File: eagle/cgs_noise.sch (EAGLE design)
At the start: 18 parts, among them IC1 TL074P, Q1 2N3906, Q2 2N3906

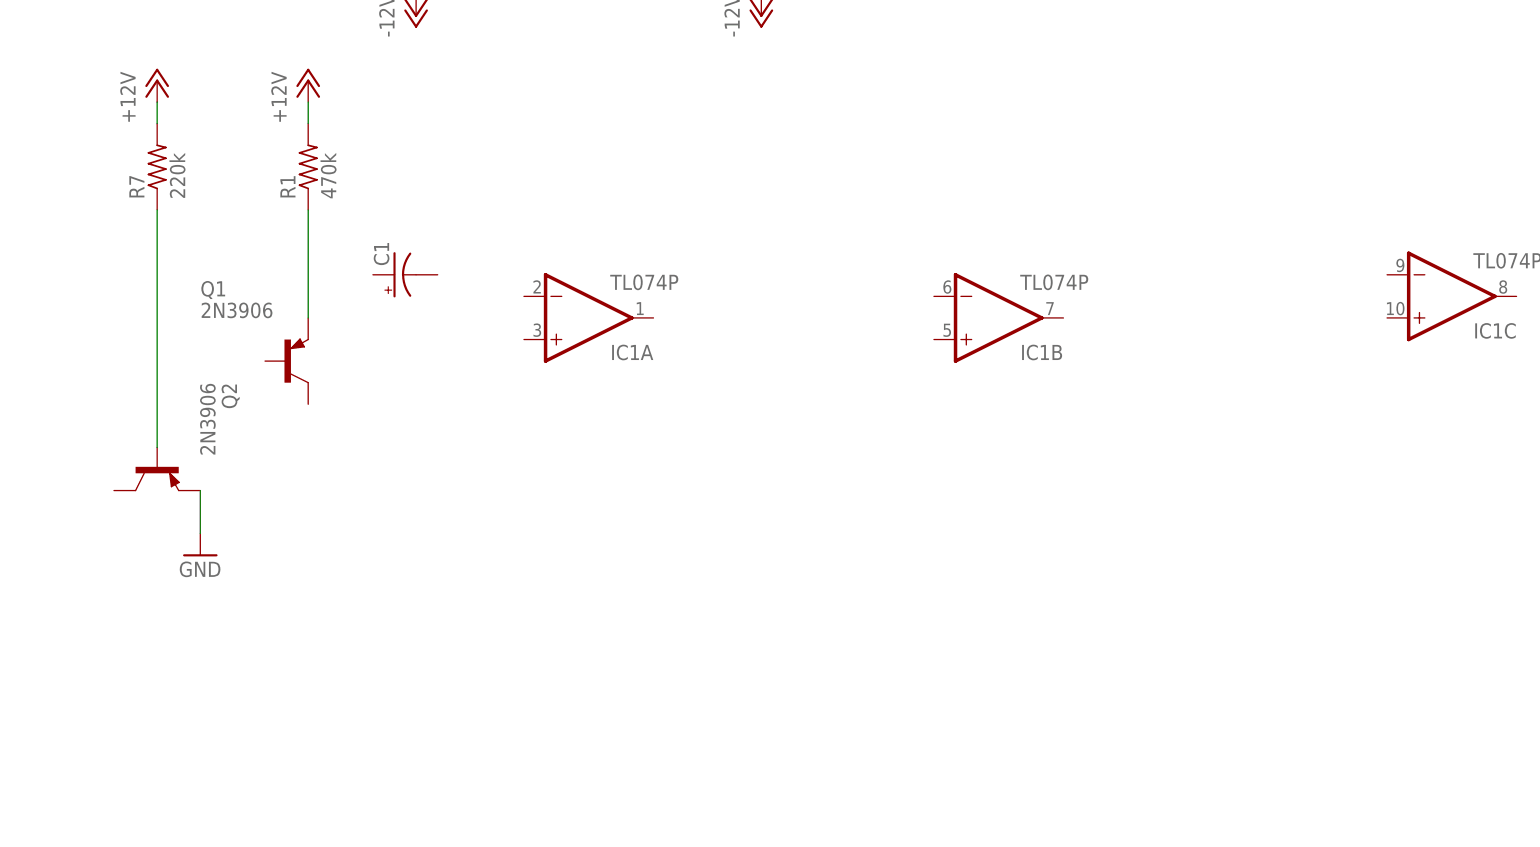
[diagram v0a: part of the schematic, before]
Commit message: initial commit
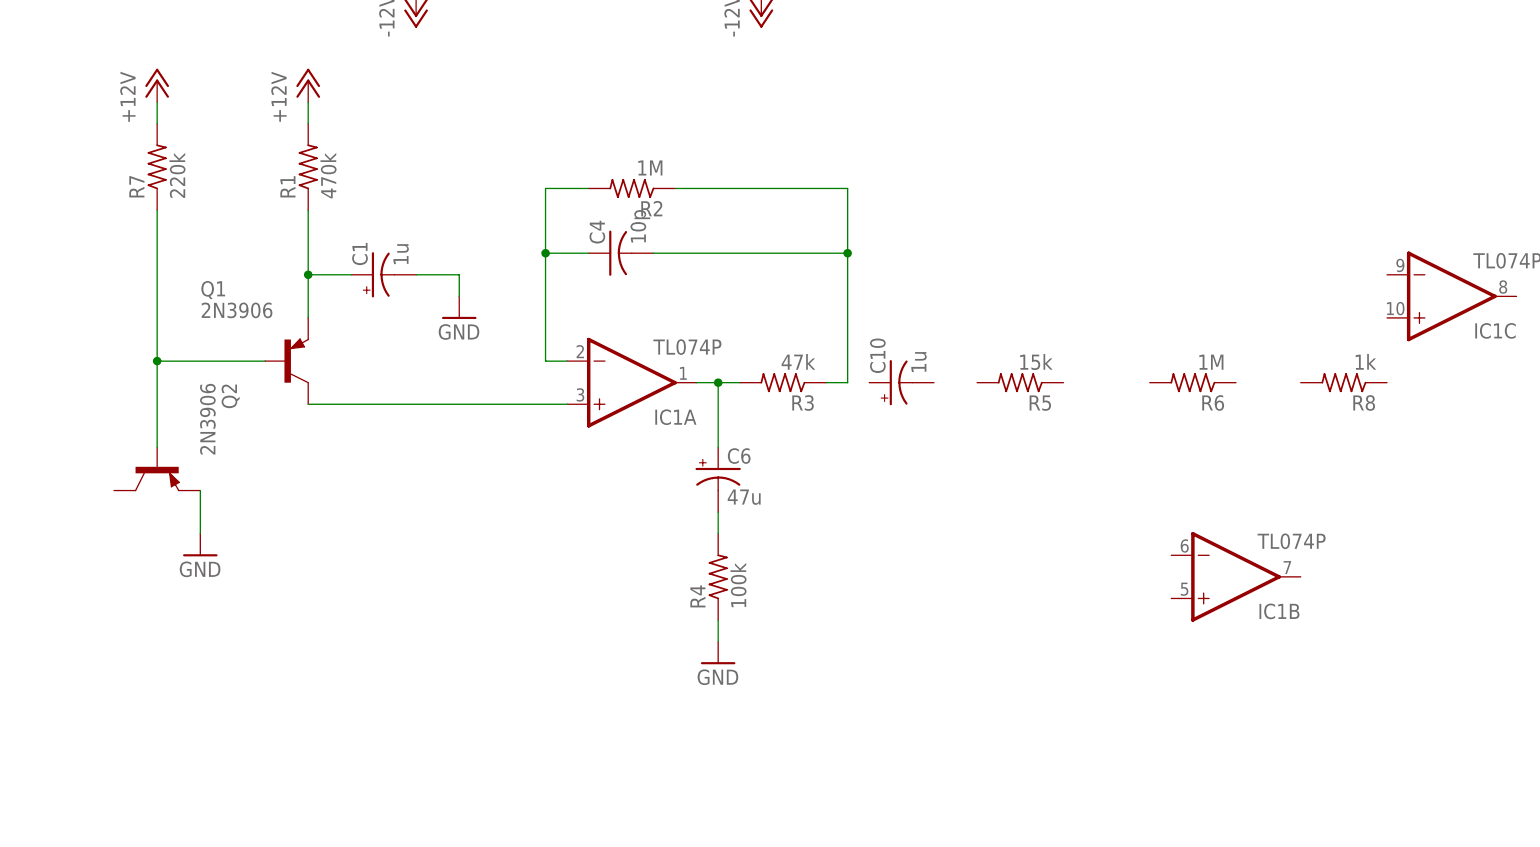
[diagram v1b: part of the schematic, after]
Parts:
- added C10: 1u, rcl:CPOL-USB45181A
- added C4: 10p, rcl:C-US050-024X044
- added C6: 47u, rcl:CPOL-USB45181A
- added R2, R6: 1M, rcl:R-US_0207/10
- added R3: 47k, rcl:R-US_0207/10
- added R4: 100k, rcl:R-US_0207/10
- added R5: 15k, rcl:R-US_0207/10
- added R8: 1k, rcl:R-US_0207/10
- C1: value (none) -> 1u
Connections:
- new net N$3: IC1A.+IN, Q1.C
- new net N$4: C6.+, IC1A.OUT, R3.2
- new net N$5: C6.-, R4.2
- new net N$6: C4.2, R2.1, R3.1
- new net N$7: C4.1, IC1A.-IN, R2.2
- net GND: now also C1.-, R4.1
- net N$1: now also C1.+
- net N$2: now also Q1.B
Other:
- moved on the sheet: C1, IC1A, IC1B
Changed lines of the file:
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@@
 <part name="Q2" library="transistor-pnp" deviceset="2N3906" device=""/>
 <part name="GND2" library="supply1" deviceset="GND" device=""/>
-<part name="C1" library="rcl" deviceset="CPOL-US" device="B45181A"/>
+<part name="C1" library="rcl" deviceset="CPOL-US" device="B45181A" value="1u"/>
+<part name="GND3" library="supply1" deviceset="GND" device=""/>
+<part name="R2" library="rcl" deviceset="R-US_" device="0207/10" value="1M"/>
+<part name="C4" library="rcl" deviceset="C-US" device="050-024X044" value="10p"/>
+<part name="R3" library="rcl" deviceset="R-US_" device="0207/10" value="47k"/>
+<part name="C6" library="rcl" deviceset="CPOL-US" device="B45181A" value="47u"/>
+<part name="R4" library="rcl" deviceset="R-US_" device="0207/10" value="100k"/>
+<part name="GND4" library="supply1" deviceset="GND" device=""/>
+<part name="C10" library="rcl" deviceset="CPOL-US" device="B45181A" value="1u"/>
+<part name="R5" library="rcl" deviceset="R-US_" device="0207/10" value="15k"/>
+<part name="R6" library="rcl" deviceset="R-US_" device="0207/10" value="1M"/>
+<part name="R8" library="rcl" deviceset="R-US_" device="0207/10" value="1k"/>
 </parts>
 <sheets>
@@
 <instance part="PN" gate="G$1" x="175.26" y="81.28" rot="R180"/>
 <instance part="GATE" gate="G$1" x="172.72" y="-5.08" rot="R180"/>
-<instance part="IC1" gate="A" x="-7.62" y="63.5" rot="MR180"/>
-<instance part="IC1" gate="B" x="40.64" y="63.5" rot="MR180"/>
+<instance part="IC1" gate="A" x="-2.54" y="55.88" rot="MR180"/>
+<instance part="IC1" gate="B" x="68.58" y="33.02" rot="MR180"/>
 <instance part="IC1" gate="C" x="93.98" y="66.04" rot="MR180"/>
 <instance part="IC1" gate="D" x="134.62" y="66.04" rot="MR180"/>
@@
 <instance part="Q2" gate="G$1" x="-58.42" y="45.72" rot="R270"/>
 <instance part="GND2" gate="1" x="-53.34" y="35.56"/>
-<instance part="C1" gate="G$1" x="-30.48" y="68.58" rot="R90"/>
+<instance part="C1" gate="G$1" x="-33.02" y="68.58" rot="R90"/>
+<instance part="GND3" gate="1" x="-22.86" y="63.5"/>
+<instance part="R2" gate="G$1" x="-2.54" y="78.74" rot="R180"/>
+<instance part="C4" gate="G$1" x="-5.08" y="71.12" rot="R90"/>
+<instance part="R3" gate="G$1" x="15.24" y="55.88" rot="R180"/>
+<instance part="C6" gate="G$1" x="7.62" y="45.72"/>
+<instance part="R4" gate="G$1" x="7.62" y="33.02" rot="R90"/>
+<instance part="GND4" gate="1" x="7.62" y="22.86"/>
+<instance part="C10" gate="G$1" x="27.94" y="55.88" rot="R90"/>
+<instance part="R5" gate="G$1" x="43.18" y="55.88" rot="R180"/>
+<instance part="R6" gate="G$1" x="63.5" y="55.88" rot="R180"/>
+<instance part="R8" gate="G$1" x="81.28" y="55.88" rot="R180"/>
 </instances>
 <busses>
@@
 <wire x1="-53.34" y1="38.1" x2="-53.34" y2="43.18" width="0.1524" layer="91"/>
 </segment>
+<segment>
+<pinref part="C1" gate="G$1" pin="-"/>
+<pinref part="GND3" gate="1" pin="GND"/>
+<wire x1="-27.94" y1="68.58" x2="-22.86" y2="68.58" width="0.1524" layer="91"/>
+<wire x1="-22.86" y1="68.58" x2="-22.86" y2="66.04" width="0.1524" layer="91"/>
+</segment>
+<segment>
+<pinref part="R4" gate="G$1" pin="1"/>
+<pinref part="GND4" gate="1" pin="GND"/>
+<wire x1="7.62" y1="27.94" x2="7.62" y2="25.4" width="0.1524" layer="91"/>
+</segment>
 </net>
 <net name="+12V" class="0">
@@
 <pinref part="R1" gate="G$1" pin="1"/>
 <pinref part="Q1" gate="G$1" pin="E"/>
-<wire x1="-40.64" y1="76.2" x2="-40.64" y2="63.5" width="0.1524" layer="91"/>
+<wire x1="-40.64" y1="76.2" x2="-40.64" y2="68.58" width="0.1524" layer="91"/>
+<pinref part="C1" gate="G$1" pin="+"/>
+<wire x1="-40.64" y1="68.58" x2="-40.64" y2="63.5" width="0.1524" layer="91"/>
+<wire x1="-35.56" y1="68.58" x2="-40.64" y2="68.58" width="0.1524" layer="91"/>
+<junction x="-40.64" y="68.58"/>
 </segment>
 </net>
@@
 <pinref part="R7" gate="G$1" pin="1"/>
 <pinref part="Q2" gate="G$1" pin="B"/>
-<wire x1="-58.42" y1="48.26" x2="-58.42" y2="76.2" width="0.1524" layer="91"/>
-</segment>
-</net>
+<wire x1="-58.42" y1="48.26" x2="-58.42" y2="58.42" width="0.1524" layer="91"/>
+<pinref part="Q1" gate="G$1" pin="B"/>
+<wire x1="-58.42" y1="58.42" x2="-58.42" y2="76.2" width="0.1524" layer="91"/>
+<wire x1="-45.72" y1="58.42" x2="-58.42" y2="58.42" width="0.1524" layer="91"/>
+<junction x="-58.42" y="58.42"/>
+</segment>
+</net>
+<net name="N$3" class="0">
+<segment>
+<pinref part="Q1" gate="G$1" pin="C"/>
+<pinref part="IC1" gate="A" pin="+IN"/>
+<wire x1="-40.64" y1="53.34" x2="-10.16" y2="53.34" width="0.1524" layer="91"/>
+</segment>
+</net>
+<net name="N$4" class="0">
+<segment>
+<pinref part="IC1" gate="A" pin="OUT"/>
+<pinref part="R3" gate="G$1" pin="2"/>
+<wire x1="10.16" y1="55.88" x2="7.62" y2="55.88" width="0.1524" layer="91"/>
+<pinref part="C6" gate="G$1" pin="+"/>
+<wire x1="7.62" y1="55.88" x2="5.08" y2="55.88" width="0.1524" layer="91"/>
+<wire x1="7.62" y1="48.26" x2="7.62" y2="55.88" width="0.1524" layer="91"/>
+<junction x="7.62" y="55.88"/>
+</segment>
+</net>
+<net name="N$5" class="0">
+<segment>
+<pinref part="C6" gate="G$1" pin="-"/>
+<pinref part="R4" gate="G$1" pin="2"/>
+<wire x1="7.62" y1="38.1" x2="7.62" y2="40.64" width="0.1524" layer="91"/>
+</segment>
+</net>
+<net name="N$6" class="0">
+<segment>
+<pinref part="R3" gate="G$1" pin="1"/>
+<wire x1="20.32" y1="55.88" x2="22.86" y2="55.88" width="0.1524" layer="91"/>
+<wire x1="22.86" y1="55.88" x2="22.86" y2="71.12" width="0.1524" layer="91"/>
+<pinref part="R2" gate="G$1" pin="1"/>
+<wire x1="22.86" y1="71.12" x2="22.86" y2="78.74" width="0.1524" layer="91"/>
+<wire x1="22.86" y1="78.74" x2="2.54" y2="78.74" width="0.1524" layer="91"/>
+<pinref part="C4" gate="G$1" pin="2"/>
+<wire x1="0" y1="71.12" x2="22.86" y2="71.12" width="0.1524" layer="91"/>
+<junction x="22.86" y="71.12"/>
+</segment>
+</net>
+<net name="N$7" class="0">
+<segment>
+<pinref part="R2" gate="G$1" pin="2"/>
+<wire x1="-7.62" y1="78.74" x2="-12.7" y2="78.74" width="0.1524" layer="91"/>
+<wire x1="-12.7" y1="78.74" x2="-12.7" y2="71.12" width="0.1524" layer="91"/>
+<pinref part="IC1" gate="A" pin="-IN"/>
+<wire x1="-12.7" y1="71.12" x2="-12.7" y2="58.42" width="0.1524" layer="91"/>
+<wire x1="-12.7" y1="58.42" x2="-10.16" y2="58.42" width="0.1524" layer="91"/>
+<pinref part="C4" gate="G$1" pin="1"/>
+<wire x1="-7.62" y1="71.12" x2="-12.7" y2="71.12" width="0.1524" layer="91"/>
+<junction x="-12.7" y="71.12"/>
+</segment>
+</net>

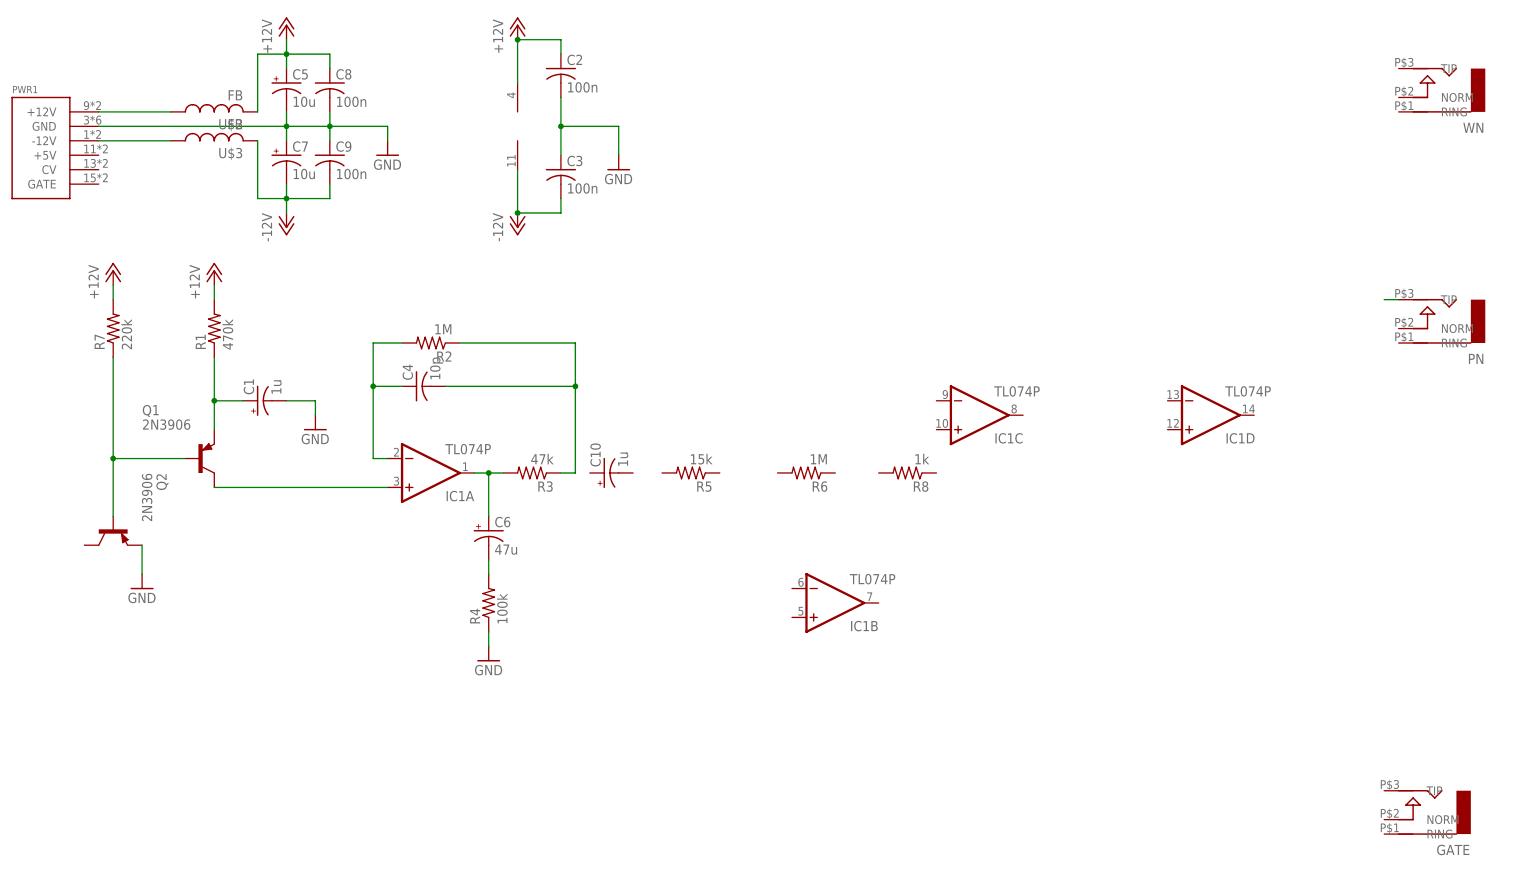
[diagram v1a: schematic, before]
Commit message: board started
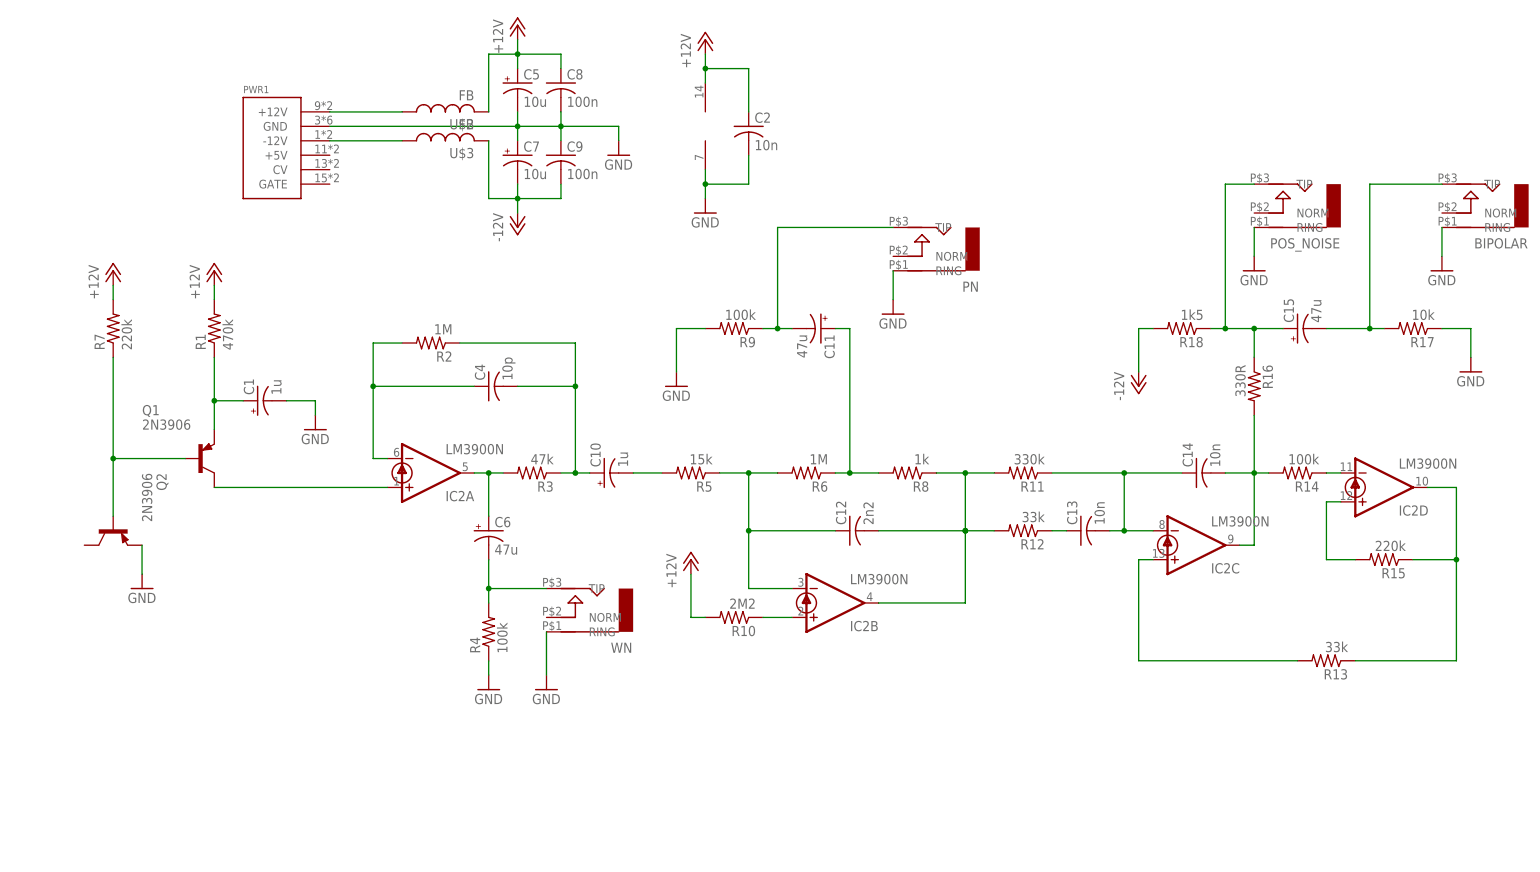
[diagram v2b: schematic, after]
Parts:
- removed C3: 100n, rcl:C-US050-024X044
- removed GATE: AUDIO-JACK, erthenvar:AUDIO-JACK
- removed IC1: TL074P, linear:TL074P
- added BIPOLAR, POS_NOISE: AUDIO-JACK, erthenvar:AUDIO-JACK
- added C11, C15: 47u, rcl:CPOL-USB45181A
- added C12: 2n2, rcl:C-US050-024X044
- added C13, C14: 10n, rcl:C-US050-024X044
- added IC2: LM3900N, linear:LM3900N
- added R10: 2M2, rcl:R-US_0207/10
- added R11: 330k, rcl:R-US_0207/10
- added R12, R13: 33k, rcl:R-US_0207/10
- added R14, R9: 100k, rcl:R-US_0207/10
- added R15: 220k, rcl:R-US_0207/10
- added R16: 330R, rcl:R-US_0207/10
- added R17: 10k, rcl:R-US_0207/10
- added R18: 1k5, rcl:R-US_0207/10
- C2: value 100n -> 10n
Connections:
- new net N$10: C11.+, R6.1, R8.2
- new net N$12: C12.2, IC2B.OUT, R11.2, R12.2, R8.1
- new net N$13: IC2C.+IN, R13.2
- new net N$14: IC2B.+IN, R10.1
- new net N$15: C14.2, IC2C.OUT, R14.2, R16.2
- new net N$16: C13.2, C14.1, IC2C.-IN, R11.1
- new net N$17: C13.1, R12.1
- new net N$19: IC2D.-IN, R14.1
- new net N$20: IC2D.OUT, R13.1, R15.1
- new net N$21: IC2D.+IN, R15.2
- new net N$22: BIPOLAR.TIP, C15.-, R17.2
- new net N$23: C15.+, POS_NOISE.TIP, R16.1, R18.1
- new net N$8: C10.-, R5.2
- new net N$9: C12.1, IC2B.-IN, R5.1, R6.2
- net +12V: now also IC2P.V+, R10.2; no longer IC1P.V+
- net -12V: now also R18.2; no longer C3.2, IC1P.V-
- net GND: now also BIPOLAR.RING, IC2P.GND, PN.RING, POS_NOISE.RING, R17.1, R9.2, WN.RING; no longer C3.1
- net N$3: now also IC2A.+IN; no longer IC1A.+IN
- net N$4: now also IC2A.OUT; no longer IC1A.OUT
- net N$5: now also WN.TIP
- net N$51: now also C11.-, R9.1
- net N$6: now also C10.+
- net N$7: now also IC2A.-IN; no longer IC1A.-IN
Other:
- moved on the sheet: C2, C4, C5, C7, C8, C9, PN, PWR1, R4, U$2, U$3, WN

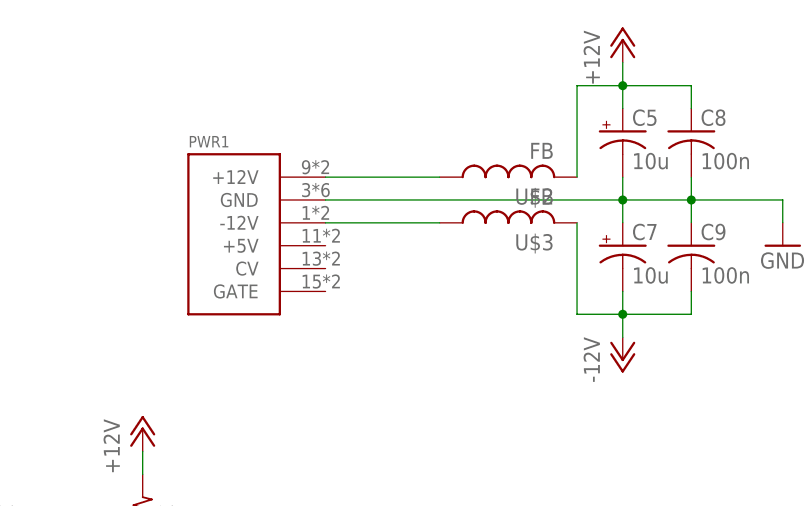
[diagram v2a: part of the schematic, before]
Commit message: gcode
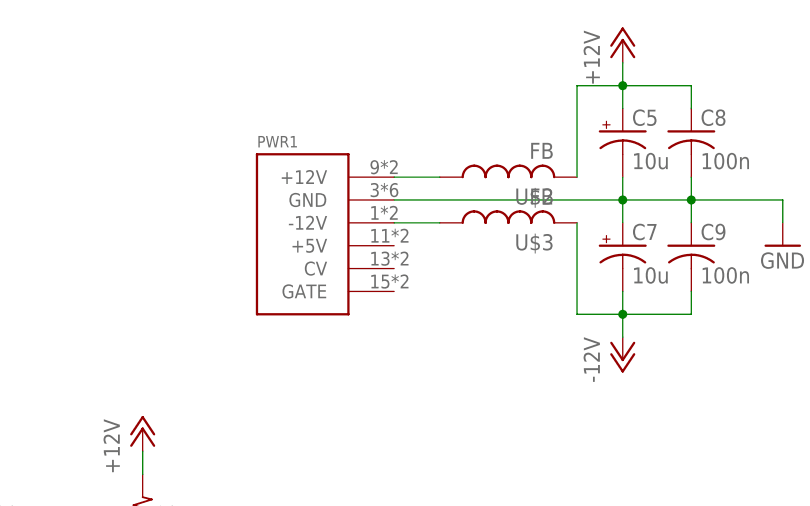
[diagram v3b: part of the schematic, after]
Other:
- moved on the sheet: PWR1
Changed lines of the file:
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@@
 <?xml version="1.0" encoding="utf-8"?>
 <!DOCTYPE eagle SYSTEM "eagle.dtd">
-<eagle version="7.2.0">
+<eagle version="7.1.0">
 <drawing>
 <settings>
@@
 <instances>
 <instance part="R7" gate="G$1" x="-58.42" y="81.28" rot="R90"/>
-<instance part="PWR1" gate="G$1" x="-30.48" y="114.3"/>
+<instance part="PWR1" gate="G$1" x="-22.86" y="114.3"/>
 <instance part="U$2" gate="G$1" x="0" y="119.38" rot="R90"/>
 <instance part="U$3" gate="G$1" x="0" y="114.3" rot="R90"/>
@@
 <pinref part="PWR1" gate="G$1" pin="GND"/>
 <pinref part="GND6" gate="1" pin="GND"/>
-<wire x1="-20.32" y1="116.84" x2="12.7" y2="116.84" width="0.1524" layer="91"/>
+<wire x1="-12.7" y1="116.84" x2="12.7" y2="116.84" width="0.1524" layer="91"/>
 <wire x1="12.7" y1="116.84" x2="20.32" y2="116.84" width="0.1524" layer="91"/>
 <wire x1="20.32" y1="116.84" x2="30.48" y2="116.84" width="0.1524" layer="91"/>
@@
 <pinref part="PWR1" gate="G$1" pin="+12V"/>
 <pinref part="U$2" gate="G$1" pin="1"/>
-<wire x1="-20.32" y1="119.38" x2="-7.62" y2="119.38" width="0.1524" layer="91"/>
+<wire x1="-12.7" y1="119.38" x2="-7.62" y2="119.38" width="0.1524" layer="91"/>
 </segment>
 </net>
@@
 <pinref part="PWR1" gate="G$1" pin="-12V"/>
 <pinref part="U$3" gate="G$1" pin="1"/>
-<wire x1="-20.32" y1="114.3" x2="-7.62" y2="114.3" width="0.1524" layer="91"/>
-</segment>
-</net>
+<wire x1="-12.7" y1="114.3" x2="-7.62" y2="114.3" width="0.1524" layer="91"/>
+</segment>
+</net>
